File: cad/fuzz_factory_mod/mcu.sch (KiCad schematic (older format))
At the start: 20 parts, among them J201 Conn_MCU_SWD, U201 STM32F303VCTx, Y201 Resonator_Small

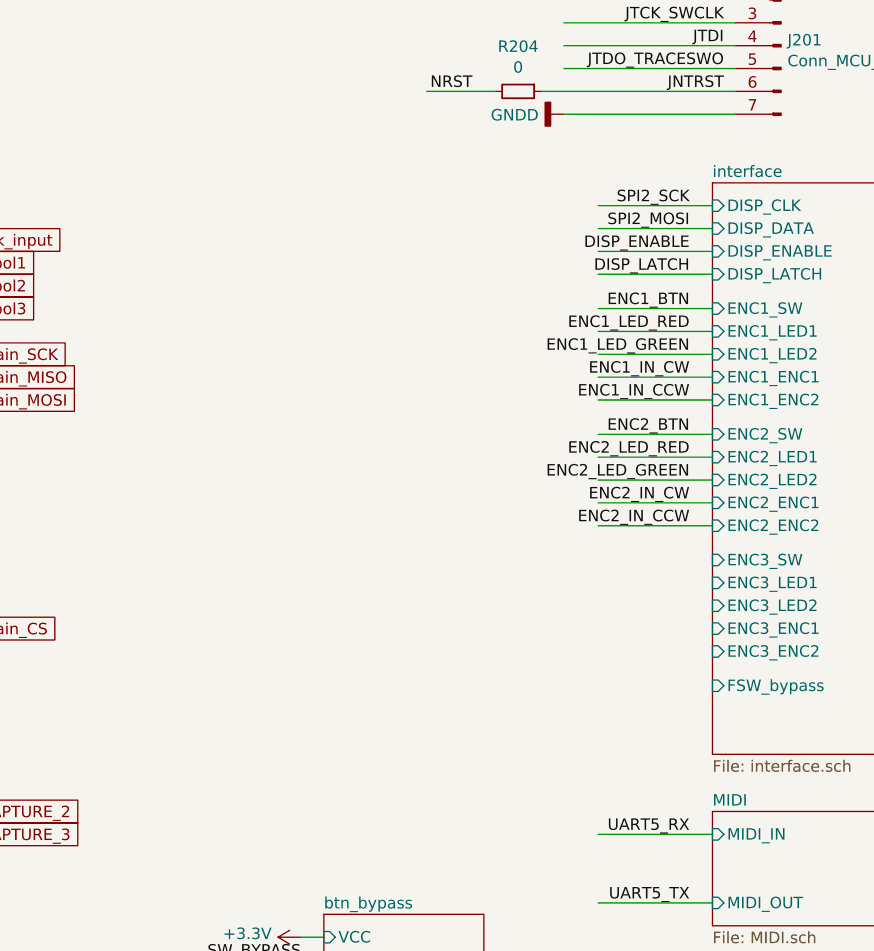
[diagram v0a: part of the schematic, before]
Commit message: Commit pre- board separation.
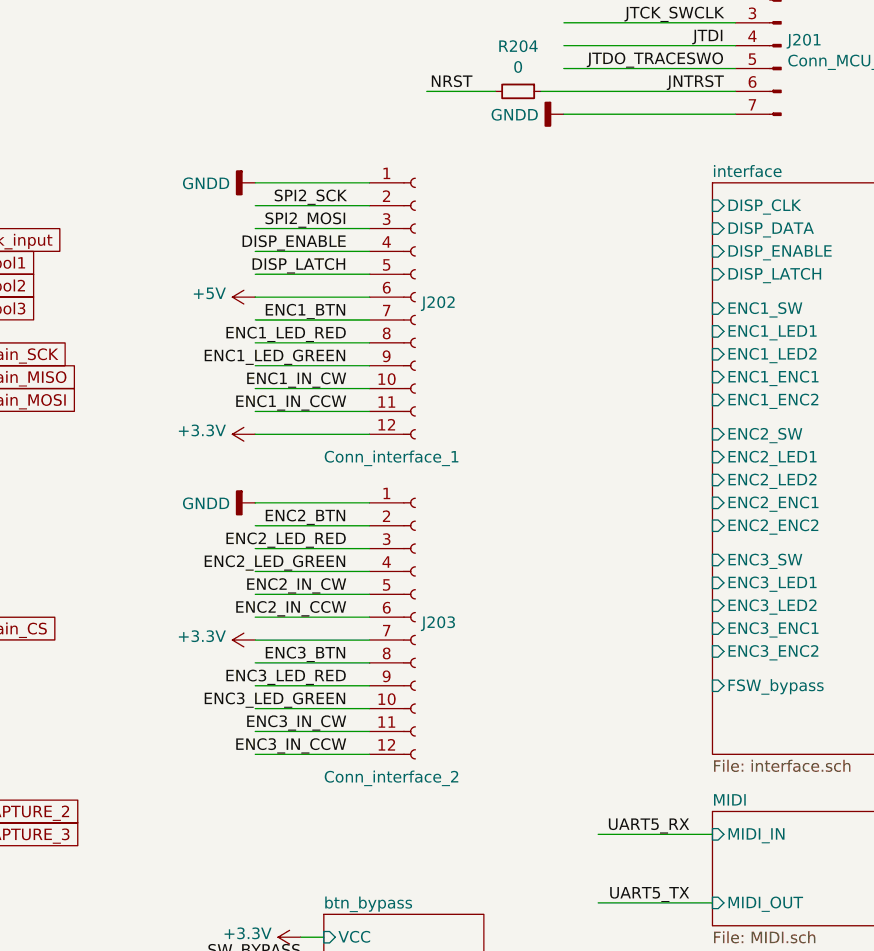
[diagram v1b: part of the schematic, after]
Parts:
- added J202: Conn_interface_1, Pin_Headers:Pin_Header_Straight_1x12_Pitch2.54mm_SMD_Pin1Left, symbol Connector:Conn_01x12_Female
- added J203: Conn_interface_2, Pin_Headers:Pin_Header_Straight_1x12_Pitch2.54mm_SMD_Pin1Left, symbol Connector:Conn_01x12_Female
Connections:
- net labels added: +5V, ENC3_BTN, ENC3_IN_CCW, ENC3_IN_CW, ENC3_LED_GREEN, ENC3_LED_RED
- wire segments 168 -> 178
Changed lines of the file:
@@
 F21 "ENC3_ENC2" I L 10000 3550 50
 $EndSheet
-Text Label 9900 1600 2    50   ~ 0
+Text Label 8400 1600 2    50   ~ 0
 SPI2_SCK
-Text Label 9900 1700 2    50   ~ 0
+Text Label 8400 1700 2    50   ~ 0
 SPI2_MOSI
 Wire Wire Line
-	10000 1600 9500 1600
-Wire Wire Line
-	10000 1700 9500 1700
-Text Label 9900 2700 2    50   ~ 0
+	8500 1600 8000 1600
+Wire Wire Line
+	8500 1700 8000 1700
+Text Label 8400 3100 2    50   ~ 0
 ENC2_LED_RED
-Text Label 9900 2800 2    50   ~ 0
+Text Label 8400 3200 2    50   ~ 0
 ENC2_LED_GREEN
-Text Label 9900 2600 2    50   ~ 0
+Text Label 8400 3000 2    50   ~ 0
 ENC2_BTN
-Text Label 9900 2900 2    50   ~ 0
+Text Label 8400 3300 2    50   ~ 0
 ENC2_IN_CW
-Text Label 9900 2050 2    50   ~ 0
+Text Label 8400 2100 2    50   ~ 0
 ENC1_BTN
-Text Label 9900 2350 2    50   ~ 0
+Text Label 8400 2400 2    50   ~ 0
 ENC1_IN_CW
-Text Label 9900 2450 2    50   ~ 0
+Text Label 8400 2500 2    50   ~ 0
 ENC1_IN_CCW
-Text Label 9900 2150 2    50   ~ 0
+Text Label 8400 2200 2    50   ~ 0
 ENC1_LED_RED
-Text Label 9900 2250 2    50   ~ 0
+Text Label 8400 2300 2    50   ~ 0
 ENC1_LED_GREEN
-Text Label 9900 3000 2    50   ~ 0
+Text Label 8400 3400 2    50   ~ 0
 ENC2_IN_CCW
 Wire Wire Line
-	10000 2050 9500 2050
-Wire Wire Line
-	10000 2150 9500 2150
-Wire Wire Line
-	10000 2250 9500 2250
-Wire Wire Line
-	10000 2350 9500 2350
-Wire Wire Line
-	10000 2450 9500 2450
-Wire Wire Line
-	10000 2600 9500 2600
-Wire Wire Line
-	10000 2700 9500 2700
-Wire Wire Line
-	10000 2800 9500 2800
-Wire Wire Line
-	10000 2900 9500 2900
-Wire Wire Line
-	10000 3000 9500 3000
+	8500 2100 8000 2100
+Wire Wire Line
+	8500 2200 8000 2200
+Wire Wire Line
+	8500 2300 8000 2300
+Wire Wire Line
+	8500 2400 8000 2400
+Wire Wire Line
+	8500 2500 8000 2500
+Wire Wire Line
+	8500 3000 8000 3000
+Wire Wire Line
+	8500 3100 8000 3100
+Wire Wire Line
+	8500 3200 8000 3200
+Wire Wire Line
+	8500 3300 8000 3300
+Wire Wire Line
+	8500 3400 8000 3400
 $Sheet
 S 10000 4250 1000 500
@@
 Text Label 5450 4150 0    50   ~ 0
 DISP_LATCH
-Text Label 9900 1900 2    50   ~ 0
+Text Label 8400 1900 2    50   ~ 0
 DISP_LATCH
-Text Label 9900 1800 2    50   ~ 0
+Text Label 8400 1800 2    50   ~ 0
 DISP_ENABLE
 Wire Wire Line
-	10000 1800 9500 1800
-Wire Wire Line
-	10000 1900 9500 1900
+	8500 1800 8000 1800
+Wire Wire Line
+	8500 1900 8000 1900
 Wire Wire Line
 	5350 4150 6500 4150
@@
 Text GLabel 6500 4350 2    50   Input ~ 0
 INPUT_CAPTURE_3
+$Comp
+L Connector:Conn_01x12_Female J202
+U 1 1 5ED776C7
+P 8700 2000
+F 0 "J202" H 8728 1976 50  0000 L CNN
+F 1 "Conn_interface_1" H 8300 1300 50  0000 L CNN
+F 2 "Pin_Headers:Pin_Header_Straight_1x12_Pitch2.54mm_SMD_Pin1Left" H 8700 2000 50  0001 C CNN
+F 3 "~" H 8700 2000 50  0001 C CNN
+	1    8700 2000
+	1    0    0    -1
+$EndComp
+$Comp
+L Connector:Conn_01x12_Female J203
+U 1 1 5ED79A9E
+P 8700 3400
+F 0 "J203" H 8728 3376 50  0000 L CNN
+F 1 "Conn_interface_2" H 8300 2700 50  0000 L CNN
+F 2 "Pin_Headers:Pin_Header_Straight_1x12_Pitch2.54mm_SMD_Pin1Left" H 8700 3400 50  0001 C CNN
+F 3 "~" H 8700 3400 50  0001 C CNN
+	1    8700 3400
+	1    0    0    -1
+$EndComp
+Text Label 8400 3700 2    50   ~ 0
+ENC3_LED_RED
+Text Label 8400 3800 2    50   ~ 0
+ENC3_LED_GREEN
+Text Label 8400 3600 2    50   ~ 0
+ENC3_BTN
+Text Label 8400 3900 2    50   ~ 0
+ENC3_IN_CW
+Text Label 8400 4000 2    50   ~ 0
+ENC3_IN_CCW
+Wire Wire Line
+	8500 3600 8000 3600
+Wire Wire Line
+	8500 3700 8000 3700
+Wire Wire Line
+	8500 3800 8000 3800
+Wire Wire Line
+	8500 3900 8000 3900
+Wire Wire Line
+	8500 4000 8000 4000
+$Comp
+L power:GNDD #PWR0227
+U 1 1 5EDA6D92
+P 8000 1500
+F 0 "#PWR0227" H 8000 1250 50  0001 C CNN
+F 1 "GNDD" V 8004 1390 50  0000 R CNN
+F 2 "" H 8000 1500 50  0001 C CNN
+F 3 "" H 8000 1500 50  0001 C CNN
+	1    8000 1500
+	0    1    1    0
+$EndComp
+Wire Wire Line
+	8500 1500 8000 1500
+$Comp
+L power:GNDD #PWR0236
+U 1 1 5EDB1D7C
+P 8000 2900
+F 0 "#PWR0236" H 8000 2650 50  0001 C CNN
+F 1 "GNDD" V 8004 2790 50  0000 R CNN
+F 2 "" H 8000 2900 50  0001 C CNN
+F 3 "" H 8000 2900 50  0001 C CNN
+	1    8000 2900
+	0    1    1    0
+$EndComp
+Wire Wire Line
+	8500 2900 8000 2900
+$Comp
+L power:+3.3V #PWR0259
+U 1 1 5EDC43BD
+P 8000 2600
+F 0 "#PWR0259" H 8000 2450 50  0001 C CNN
+F 1 "+3.3V" V 8015 2728 50  0000 L CNN
+F 2 "" H 8000 2600 50  0001 C CNN
+F 3 "" H 8000 2600 50  0001 C CNN
+	1    8000 2600
+	0    -1   -1   0
+$EndComp
+Wire Wire Line
+	8000 2000 8500 2000
+$Comp
+L power:+5V #PWR0260
+U 1 1 5EDD067C
+P 8000 2000
+F 0 "#PWR0260" H 8000 1850 50  0001 C CNN
+F 1 "+5V" V 8015 2128 50  0000 L CNN
+F 2 "" H 8000 2000 50  0001 C CNN
+F 3 "" H 8000 2000 50  0001 C CNN
+	1    8000 2000
+	0    -1   -1   0
+$EndComp
+Wire Wire Line
+	8500 2600 8000 2600
+$Comp
+L power:+3.3V #PWR0261
+U 1 1 5EDDC1B4
+P 8000 3500
+F 0 "#PWR0261" H 8000 3350 50  0001 C CNN
+F 1 "+3.3V" V 8015 3628 50  0000 L CNN
+F 2 "" H 8000 3500 50  0001 C CNN
+F 3 "" H 8000 3500 50  0001 C CNN
+	1    8000 3500
+	0    -1   -1   0
+$EndComp
+Wire Wire Line
+	8500 3500 8000 3500
 $EndSCHEMATC
